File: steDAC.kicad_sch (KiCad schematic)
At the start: 17 parts

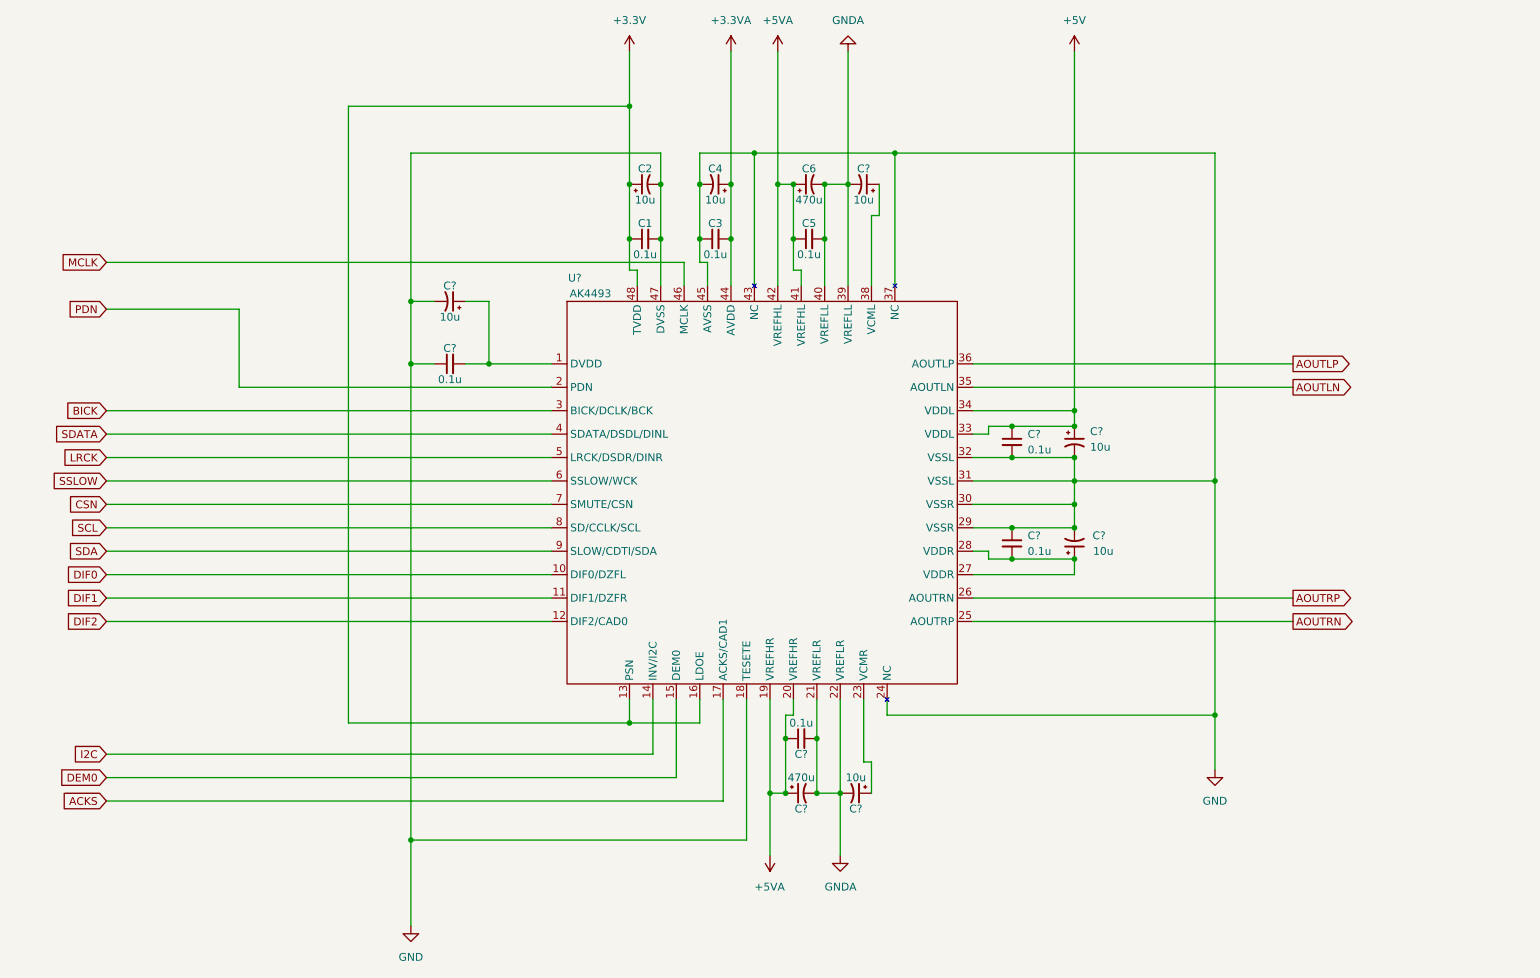
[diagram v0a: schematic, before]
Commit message: Adding Initial MCU configuration
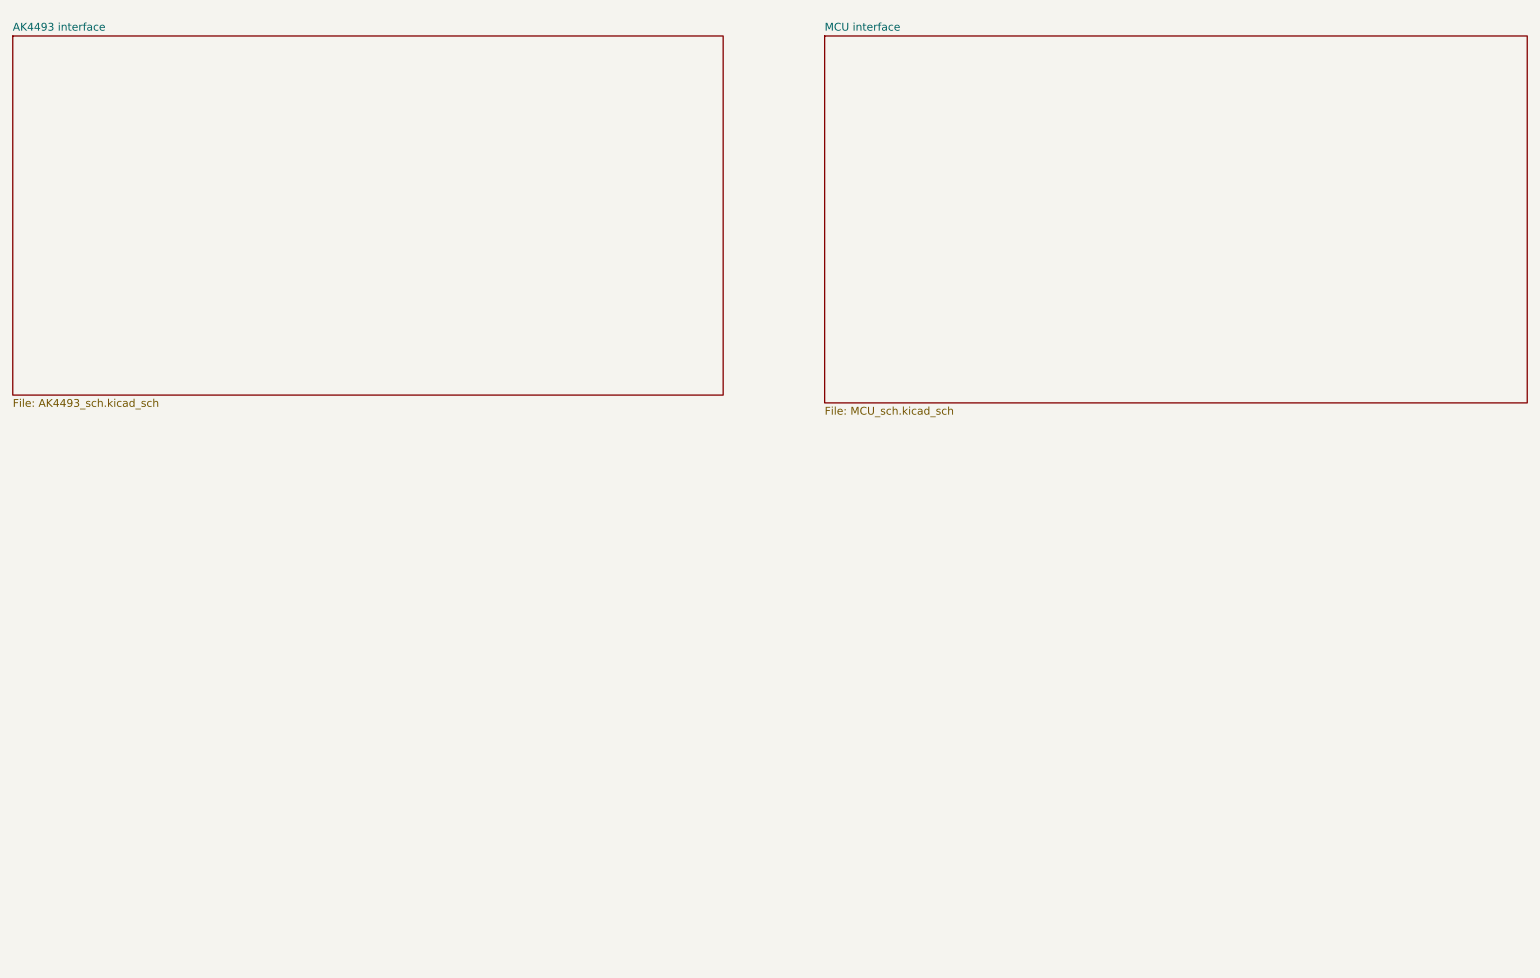
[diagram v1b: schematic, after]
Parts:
- removed C1, C3, C5, C? (x4): 0.1u, symbol Device:C_Small
- removed C2, C4, C? (x5): 10u, symbol Device:C_Polarized_Small_US
- removed C6, C?: 470u, symbol Device:C_Polarized_Small_US
- removed U?: AK4493, symbol steDAC:AK4493
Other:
- added sheet AK4493 interface (AK4493_sch.kicad_sch)
- added sheet MCU interface (MCU_sch.kicad_sch)
